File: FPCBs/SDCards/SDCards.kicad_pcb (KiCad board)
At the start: 2 copper layers, 45 x 77.4 mm, 4 parts, among them J1 SD_Card_Device, J2 SD_Card_Device, J3 SD_Card_Device, J4 SD_Card_Device

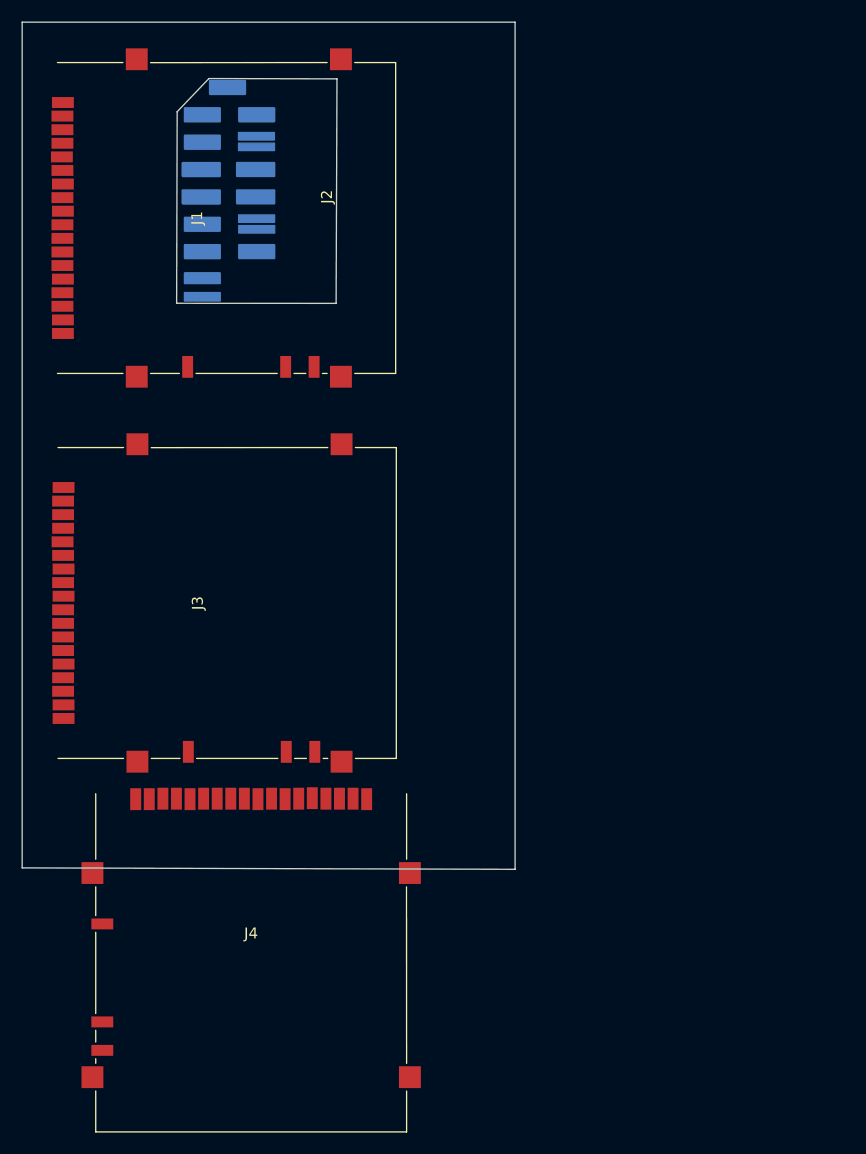
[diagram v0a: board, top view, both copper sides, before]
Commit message: Fix sd card
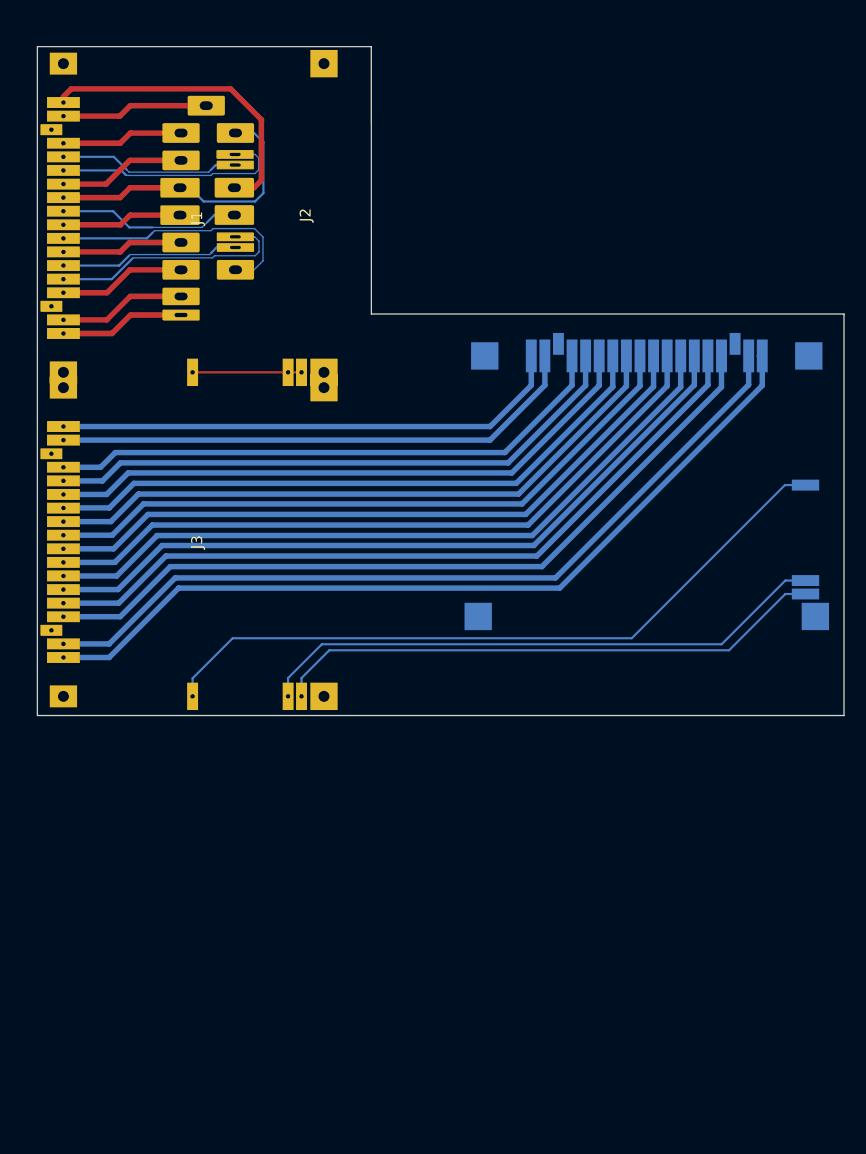
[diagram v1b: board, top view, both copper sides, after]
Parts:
- J1, J3: footprint Leica-G9ii:SD_Card_Socket_UHS-II_HTK_AXA573062 -> Leica-G9ii:SD_Card_Socket_UHS-II_Extender
- J4: moved to B.Cu
- moved J4 54.3 mm to (125.2, 107.2), turned to 180 degrees
- moved J3 5.57 mm to (86.8, 109.2)
- moved J2 2.56 mm to (80.7, 79.4)
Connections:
- J1 pad WP: (no net) -> Net-(J1-CARD_DETECT)
- J2 pad 10: Net-(J1-VSS3) -> Net-(J1-VSS1)
- J3 pad WP: (no net) -> Net-(J3-WRITE_PROTECT)
- J4 pad WP: (no net) -> Net-(J3-WRITE_PROTECT)
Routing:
- net Net-(J3-DAT1): track 0.00 -> 77.3 mm
- net Net-(J3-DAT0): track 0.00 -> 75.0 mm
- net Net-(J3-VSS2): track 0.00 -> 71.7 mm
- net Net-(J3-D1-): track 0.00 -> 69.8 mm
- net Net-(J3-D1+): track 0.00 -> 68.0 mm
- net Net-(J3-CLK): track 0.00 -> 66.4 mm
- net Net-(J3-CARD_DETECT): track 0.00 -> 65.0 mm
- net Net-(J3-Name): track 0.00 -> 64.6 mm
- net Net-(J3-VDD): track 0.00 -> 62.8 mm
- net Net-(J3-VDD2): track 0.00 -> 61.1 mm
- net Net-(J3-VSS1): track 0.00 -> 59.3 mm
- net Net-(J3-CMD): track 0.00 -> 57.6 mm
- net Net-(J3-D0+): track 0.00 -> 55.8 mm
- net Net-(J3-D0-): track 0.00 -> 54.0 mm
- net Net-(J3-WRITE_PROTECT): track 0.00 -> 52.6 mm
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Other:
- board size 45 x 77.4 mm -> 73.7 x 61.1 mm
